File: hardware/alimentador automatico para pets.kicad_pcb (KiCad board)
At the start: 2 copper layers, 96 x 90 mm, 31 parts, among them J1 Conn_01x02, J2 Conn_01x04, J3 Conn_01x03, J4 Conn_01x03, J5 Conn_01x02, J6 Conn_01x05, J7 Conn_01x02, J8 Conn_01x04, Q1 BC337, SW1 SW_Push, SW2 SW_Push, SW3 SW_Push, U1 ESP32-DEVKIT-V1, U2 HX711_module, U3 TP4056

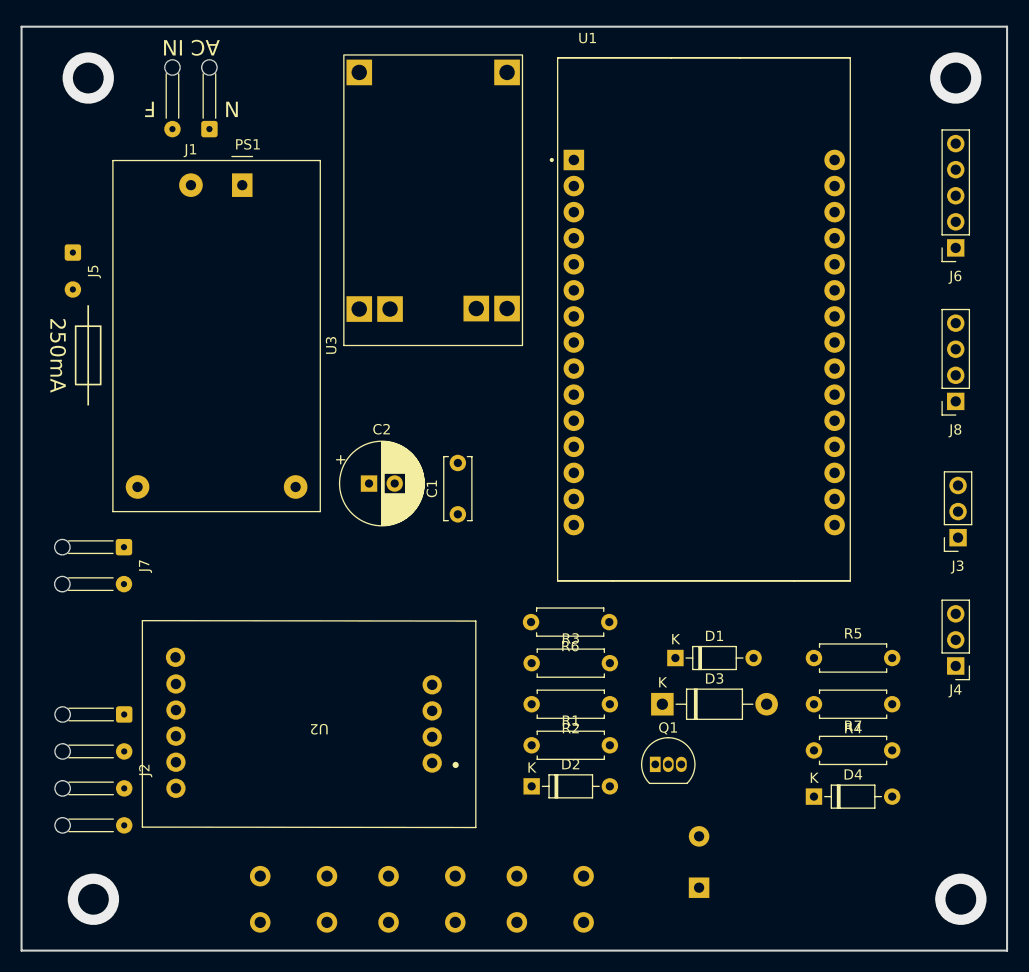
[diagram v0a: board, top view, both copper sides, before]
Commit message: place components and board roadmap #22
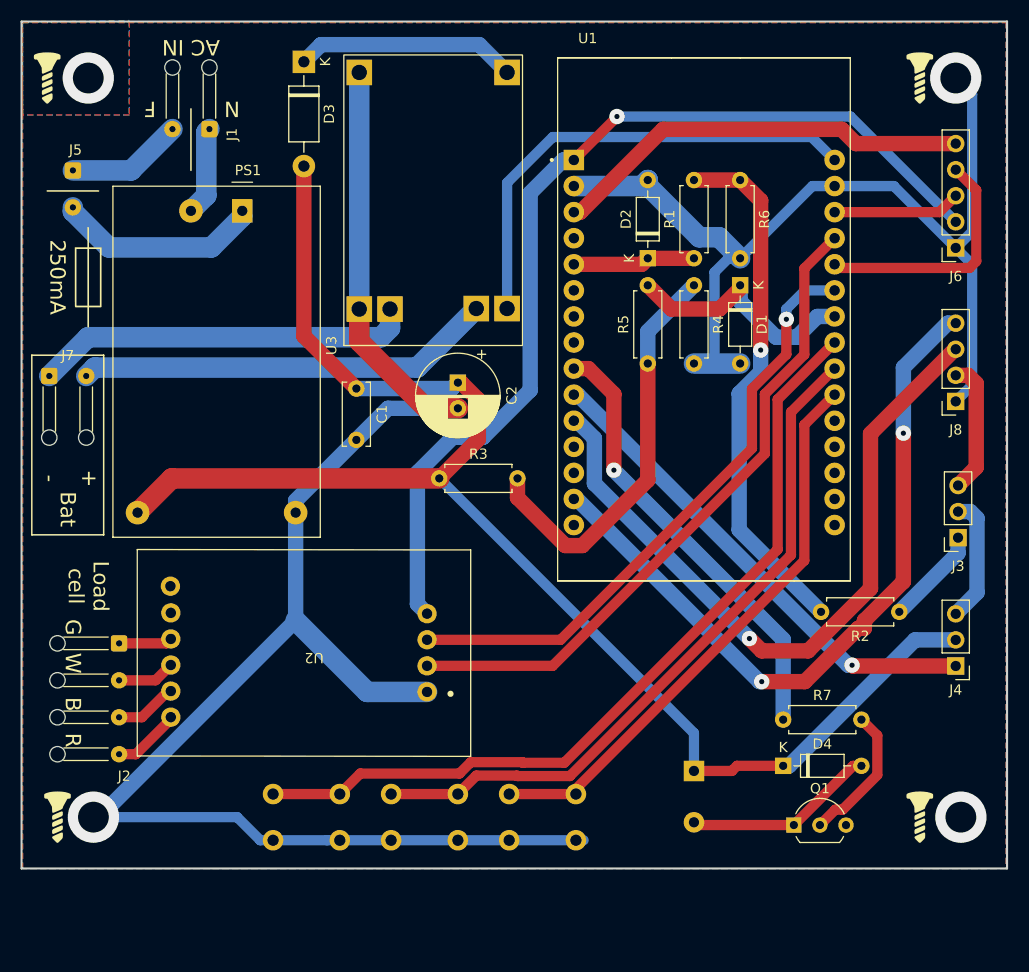
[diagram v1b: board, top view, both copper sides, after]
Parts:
- added G***: LOGO, footprint_lib:parafuso, F.Cu at (111.0, 102.0)
- added G***: LOGO, footprint_lib:parafuso, F.Cu at (27.0, 102.0)
- added G***: LOGO, footprint_lib:parafuso, F.Cu at (26.0, 30.0)
- added G***: LOGO, footprint_lib:parafuso, F.Cu at (111.0, 30.0)
- added G***: LOGO, footprint_lib:danger, B.Cu at (35.0, 40.8)
- Q1: footprint Package_TO_SOT_THT:TO-92_Inline -> Package_TO_SOT_THT:TO-92L_Inline_Wide
- moved D3 71.7 mm to (51.0, 28.4), turned to -90 degrees
- moved D2 52.7 mm to (84.5, 47.6), turned to 90 degrees
- moved R1 50.0 mm to (89.0, 47.6), turned to 90 degrees
- moved R4 45.1 mm to (89.0, 50.2), turned to -90 degrees
- moved R6 44.9 mm to (93.5, 39.9), turned to -90 degrees
- moved D1 36.9 mm to (93.5, 50.2), turned to -90 degrees
- moved R5 32.9 mm to (84.5, 57.8), turned to 90 degrees
- moved R2 29.6 mm to (109.0, 82.0)
- moved R3 20.1 mm to (64.2, 69.0)
- moved J7 18.2 mm to (26.2, 59.0), turned to 0 degrees
- moved C1 15.7 mm to (56.1, 60.2), turned to -90 degrees
- moved Q1 14.7 mm to (98.7, 102.8)
- moved SW2 14.6 mm to (66.0, 99.8)
- moved SW1 14.2 mm to (77.5, 99.8)
- moved C2 13.1 mm to (66.0, 59.7), turned to -90 degrees
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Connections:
- J7 pad 1: Net-(J7-Pad1) -> Net-(U3-Pad4)
- J7 pad 2: Net-(J7-Pad2) -> Net-(U3-Pad5)
- U3 pad 4: Net-(J7-Pad2) -> Net-(U3-Pad4)
- U3 pad 5: Net-(J7-Pad1) -> Net-(U3-Pad5)
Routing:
- net GND: track 0.00 -> 273.0 mm, vias 4 -> 3
- net /5V: track 0.00 -> 159.2 mm
- net /3V3: track 0.00 -> 96.5 mm, vias 0 -> 1
- net /BUTTON_3: track 0.00 -> 81.5 mm
- net /SCL_disp: track 0.00 -> 71.7 mm, vias 0 -> 2
- net /SDA_disp: track 0.00 -> 70.1 mm, vias 0 -> 1
- net /BUTTON_2: track 0.00 -> 68.6 mm
- net /DT: track 0.00 -> 65.3 mm
- net /SCK: track 0.00 -> 59.8 mm, vias 0 -> 1
- net /BUTTON_1: track 0.00 -> 55.8 mm
- net Net-(R1-Pad2): track 0.00 -> 51.3 mm, vias 0 -> 1
- net /sMotor: track 0.00 -> 48.1 mm, vias 0 -> 1
- net /+Vcc: track 0.00 -> 46.9 mm
- net /buzzer: track 0.00 -> 43.5 mm, vias 0 -> 1
- net /CLK_encoder: track 0.00 -> 41.1 mm
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- added copper zone on B.Cu, net (none)
- added copper zone on F.Cu, net (none)
- added copper zone on B.Cu, net GND
- added copper zone on F.Cu, net GND
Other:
- board size 96 x 90 mm -> 96 x 82.5 mm
- board text added: "+"
- board text added: "-"
- board text added: "B"
- board text added: "Bat"
- board text added: "G"
- board text added: "Load cell"
- board text added: "R"
- board text added: "W"
